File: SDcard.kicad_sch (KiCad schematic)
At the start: 21 parts, among them J1 Conn_01x04, J4 Conn_01x08, J6 Micro_SD_Card_Det_Hirose_DM3AT

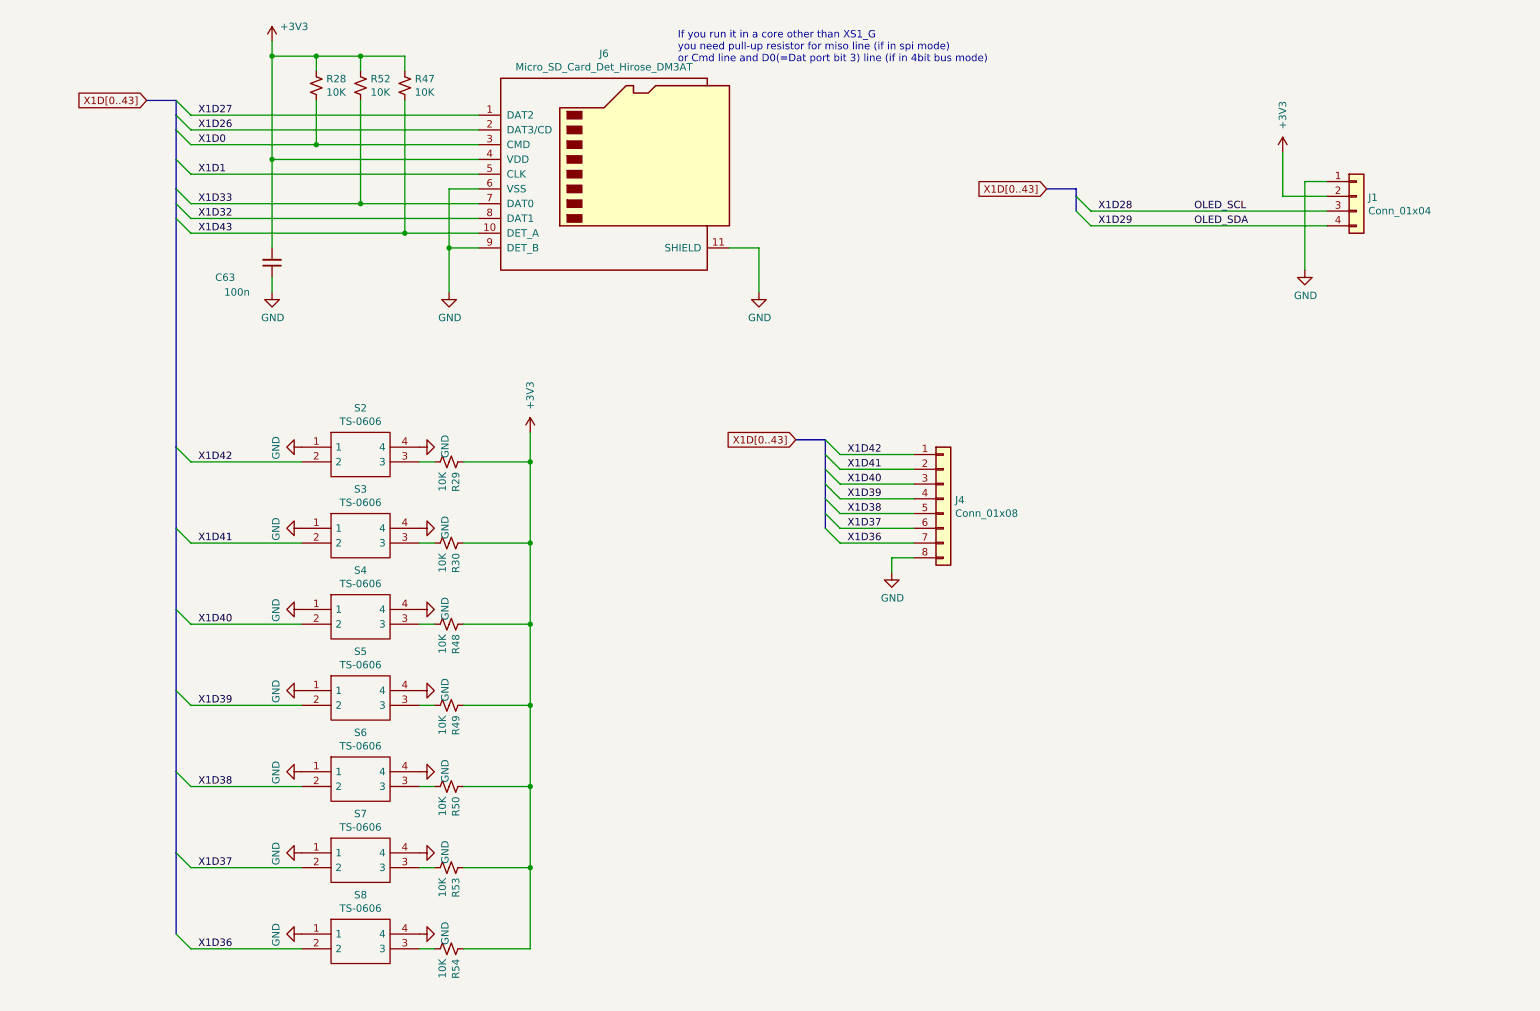
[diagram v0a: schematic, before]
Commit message: V2.0
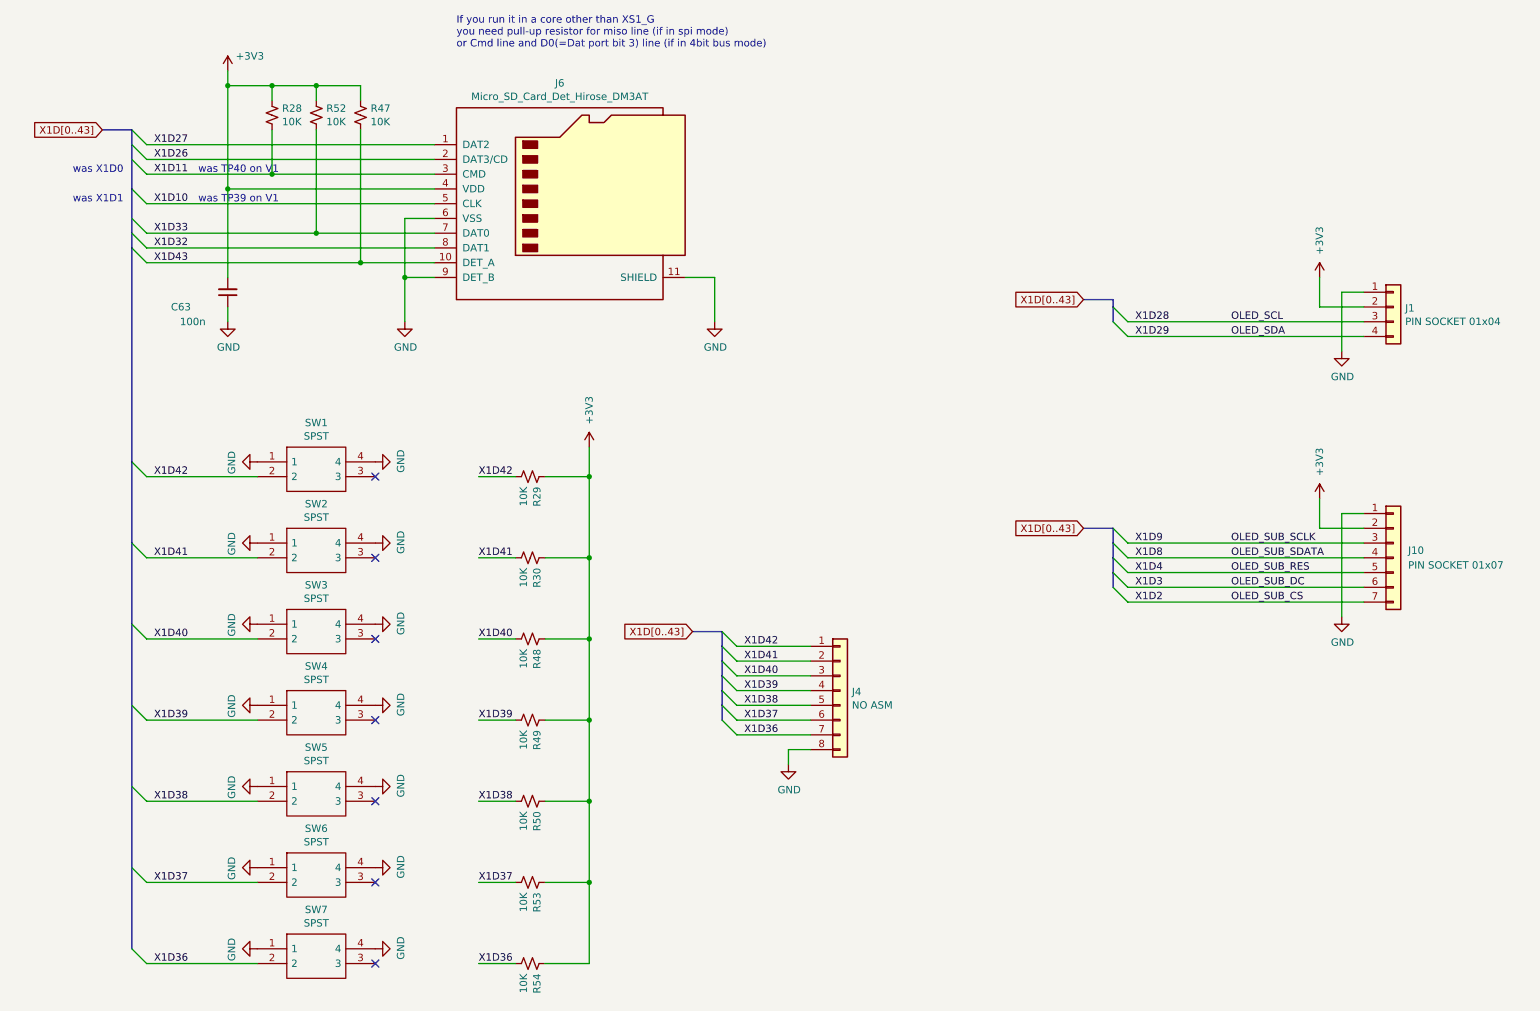
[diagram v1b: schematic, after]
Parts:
- added J10: PIN SOCKET 01x07, pretty:OLED_7pin_0.95_96X64_RGB, symbol Connector_Generic:Conn_01x07
- J1: value Conn_01x04 -> PIN SOCKET 01x04; footprint pretty:OLED_128X64 -> pretty:OLED_4pin_1.3_128X64
- J4: value Conn_01x08 -> NO ASM
- SW1: renamed from S2; value TS-0606 -> SPST; Manufacturer_Name (none) -> Cosland Co,. Ltd.; Manufacturer_Part_Number (none) -> DTS-63-N-V-RED
- SW2: renamed from S3; value TS-0606 -> SPST; Manufacturer_Name (none) -> Cosland Co,. Ltd.; Manufacturer_Part_Number (none) -> DTS-63-N-V-WHT
- SW3: renamed from S4; value TS-0606 -> SPST; Manufacturer_Name (none) -> Cosland Co,. Ltd.; Manufacturer_Part_Number (none) -> DTS-63-N-V-WHT
- SW4: renamed from S5; value TS-0606 -> SPST; Manufacturer_Name (none) -> Cosland Co,. Ltd.; Manufacturer_Part_Number (none) -> DTS-63-N-V-RED
- SW5: renamed from S6; value TS-0606 -> SPST; Manufacturer_Name (none) -> Cosland Co,. Ltd.; Manufacturer_Part_Number (none) -> DTS-63-N-V-WHT
- SW6: renamed from S7; value TS-0606 -> SPST; Manufacturer_Name (none) -> Cosland Co,. Ltd.; Manufacturer_Part_Number (none) -> DTS-63-N-V-WHT
- SW7: renamed from S8; value TS-0606 -> SPST; Manufacturer_Name (none) -> Cosland Co,. Ltd.; Manufacturer_Part_Number (none) -> DTS-63-N-V-RED
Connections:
- net +3V3: now also J10.2 (Pin_2)
- net GND: now also J10.1 (Pin_1)
- net X1D36: now also R54.2
- net X1D37: now also R53.2
- net X1D38: now also R50.2
- net X1D39: now also R49.2
- net X1D40: now also R48.2
- net X1D41: now also R30.2
- net X1D42: now also R29.2
- net at SW1.3: no longer R29.2
- net at SW2.3: no longer R30.2
- net at SW3.3: no longer R48.2
- net at SW4.3: no longer R49.2
- net at SW5.3: no longer R50.2
- net at SW6.3: no longer R53.2
- net at SW7.3: no longer R54.2
- net X1D0 renamed X1D11
- net X1D1 renamed X1D10
- new net OLED_SUB_CS: J10.7 (Pin_7)
- new net OLED_SUB_DC: J10.6 (Pin_6)
- new net OLED_SUB_RES: J10.5 (Pin_5)
- new net OLED_SUB_SCLK: J10.3 (Pin_3)
- new net OLED_SUB_SDATA: J10.4 (Pin_4)
- no-connect marks 0 -> 7
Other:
- note added: "was TP39 on V1"
- note added: "was TP40 on V1"
- note added: "was X1D0"
- note added: "was X1D1"
- moved on the sheet: C63, J1, J4, J6, R28, R29, R30, R47, R48, R49, R50, R52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
